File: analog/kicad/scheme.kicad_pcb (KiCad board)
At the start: 2 copper layers, 62.5 x 27 mm, 25 parts, among them J1 Barrel_Jack_Switch, U1 LM7805_TO220, U2 LM324

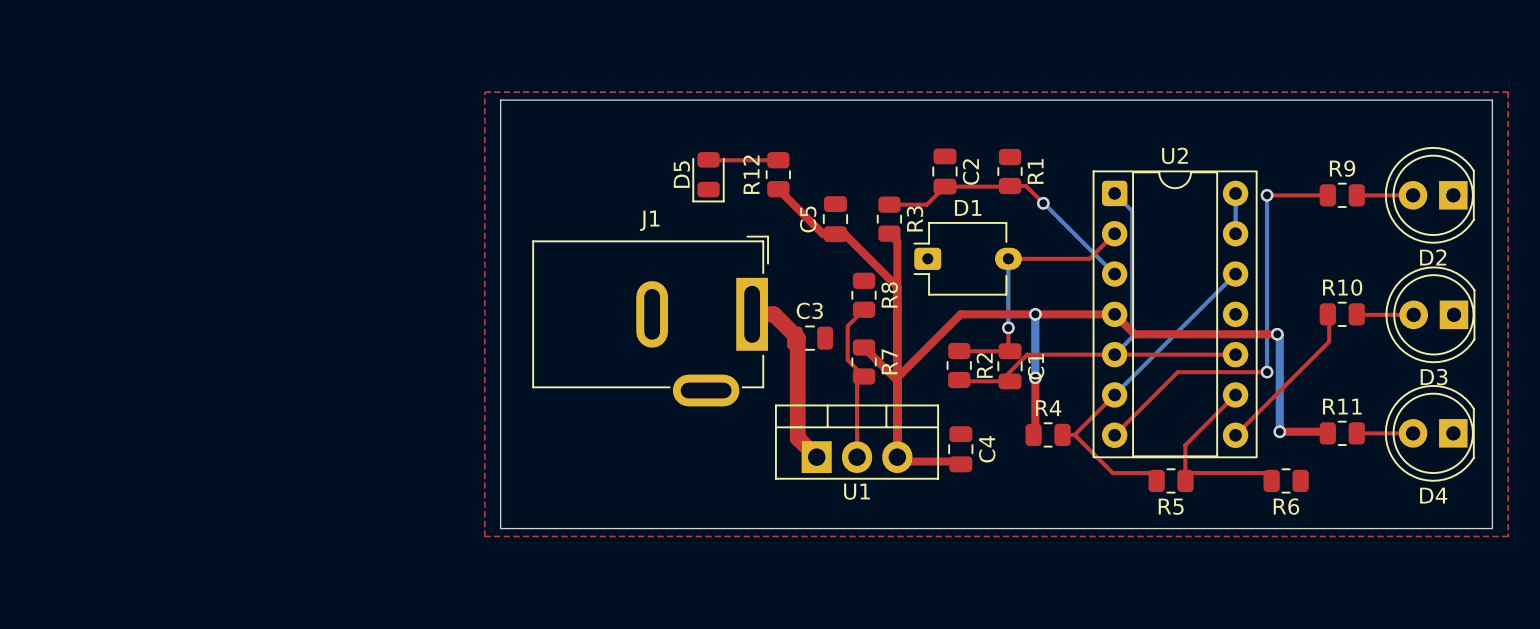
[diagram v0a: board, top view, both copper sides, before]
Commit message: pcb changes
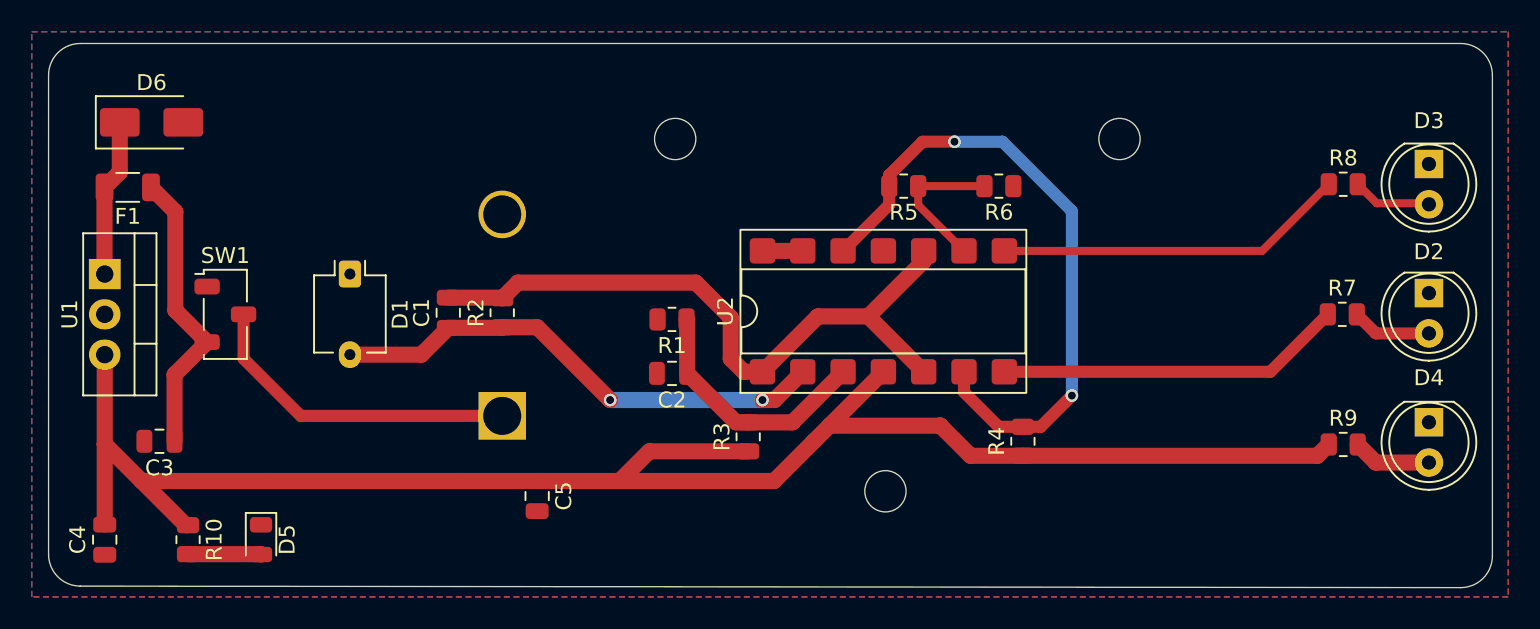
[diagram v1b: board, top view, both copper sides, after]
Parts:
- removed J1: Barrel_Jack_Switch, Connector_BarrelJack:BarrelJack_GCT_DCJ200-10-A_Horizontal
- removed the R7 at (131.4, 95.0)
- removed the R8 at (131.4, 90.8)
- added BT1: Battery_Cell 9V, Battery:BatteryHolder_Eagle_12BH611-GR, B.Cu at (108.6, 98.4)
- added D6: SMAJ13A, Diode_SMD:D_SMA, F.Cu at (86.5, 79.9)
- added F1: SMDH1206B005TF, Resistor_SMD:R_1206_3216Metric, F.Cu at (85.0, 84.0)
- added SW1: SW_Nidec_CAS-120A1, Button_Switch_SMD:Nidec_Copal_CAS-120A, F.Cu at (91.2, 92.0)
- U2: footprint Package_DIP:DIP-14_W7.62mm_Socket -> Package_DIP:DIP-14_W7.62mm_SMDSocket_SmallPads
- moved C4 54.3 mm to (83.5, 106.2), turned to -90 degrees
- moved U1 46.3 mm to (83.5, 89.5), turned to -90 degrees
- moved R10 43.7 mm to (88.8, 106.2), turned to -90 degrees
- moved C3 41.5 mm to (87.0, 100.0), turned to 180 degrees
- moved D1 36.4 mm to (99.0, 89.5), turned to -90 degrees
- moved D5 36.4 mm to (93.4, 106.2), turned to -90 degrees
- moved C1 35.6 mm to (105.2, 91.9), turned to 90 degrees
- moved R2 29.0 mm to (108.6, 91.9), turned to 90 degrees
- moved R6 25.9 mm to (139.9, 83.9)
- moved C5 25.7 mm to (110.8, 103.5), turned to -90 degrees
- moved R5 25.1 mm to (133.9, 83.9)
- moved R1 23.2 mm to (119.3, 92.3), turned to 180 degrees
- moved C2 21.4 mm to (119.3, 95.7), turned to 180 degrees
- moved U2 16.4 mm to (132.6, 91.8), turned to 90 degrees
- moved R3 16.4 mm to (124.1, 99.7), turned to 90 degrees
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- renumbered R12 to R10, R9 to R7, R10 to R8, R11 to R9
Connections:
- net /OUT renamed TIA_OUT
- net /dist2 renamed /(1.7V)
- net /dist3 renamed (2.5V)
- C2 pad 1: GND -> VGND
- C2 pad 2: /BIAS -> GND
- C3 pad 1: Net-(U1-VI) -> Net-(SW1-A)
- R1 pad 1: GND -> VGND
- R1 pad 2: /BIAS -> GND
- R3 pad 1: /BIAS -> +5V
- R3 pad 2: +5V -> VGND
- U1 pad 1: Net-(U1-VI) -> Net-(D6-A1)
- U1 pad 2: Net-(U1-GND) -> GND
- U2 pad 3: /BIAS -> VGND
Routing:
- net Net-(BT1-+): track 0.00 -> 20.6 mm
- net (2.5V): track 21.8 -> 41.6 mm, vias 0 -> 2
- net Net-(SW1-A): track 0.00 -> 18.3 mm
- net /BIAS: track 17.3 -> 0.00 mm, vias 1 -> 0
- net VGND: track 0.00 -> 15.8 mm
- net Net-(D1-A): track 16.1 -> 31.9 mm, vias 1 -> 2
- net +5V: track 95.1 -> 109.1 mm, vias 4 -> 0
- net TIA_OUT: track 29.2 -> 42.7 mm
- net Net-(R8-Pad1): track 10.1 -> 22.2 mm
- net Net-(U1-VI): track 11.5 -> 0.00 mm
- net Net-(U1-GND): track 10.4 -> 0.00 mm
- net Net-(D6-A1): track 0.00 -> 9.96 mm
- net Net-(R7-Pad1): track 26.3 -> 21.9 mm, vias 2 -> 0
- net /(1.7V): track 11.8 -> 9.45 mm
- net Net-(D2-A): track 3.63 -> 5.04 mm
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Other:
- board size 62.5 x 27 mm -> 91 x 34.3 mm
